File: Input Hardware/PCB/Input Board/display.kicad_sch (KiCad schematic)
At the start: 10 parts

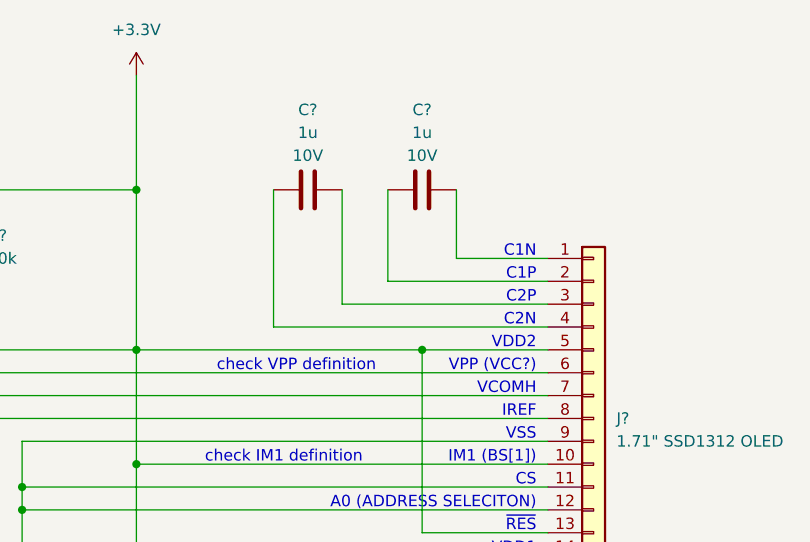
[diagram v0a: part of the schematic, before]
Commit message: images and pcb stuff
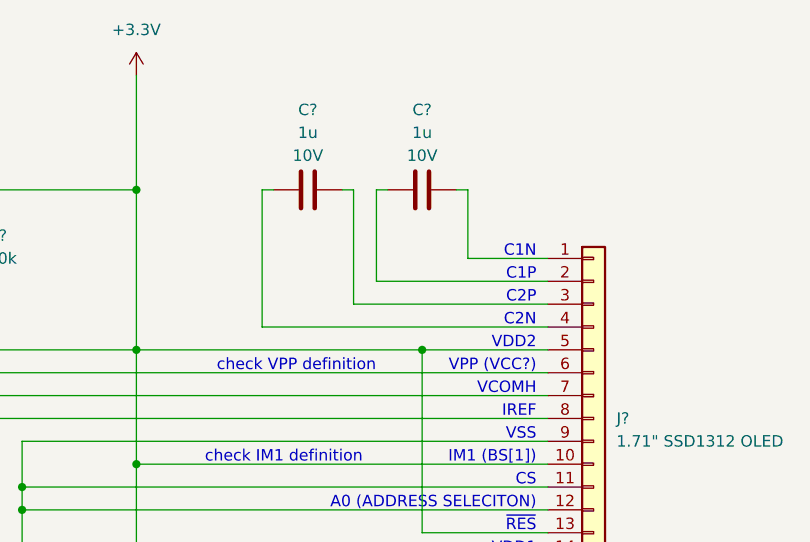
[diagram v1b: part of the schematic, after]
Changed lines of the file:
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@@
+	(wire
+		(pts
+			(xy 140.97 63.5) (xy 142.24 63.5)
+		)
+		(stroke
+			(width 0)
+			(type default)
+		)
+	)
 	(wire
 		(pts
@@
 	(wire
 		(pts
-			(xy 172.72 73.66) (xy 154.94 73.66)
+			(xy 172.72 73.66) (xy 153.67 73.66)
+		)
+		(stroke
+			(width 0)
+			(type default)
+		)
+	)
+	(wire
+		(pts
+			(xy 163.83 63.5) (xy 162.56 63.5)
 		)
 		(stroke
@@
 	(wire
 		(pts
-			(xy 162.56 71.12) (xy 172.72 71.12)
+			(xy 163.83 71.12) (xy 172.72 71.12)
+		)
+		(stroke
+			(width 0)
+			(type default)
+		)
+	)
+	(wire
+		(pts
+			(xy 153.67 63.5) (xy 154.94 63.5)
 		)
 		(stroke
@@
 	(wire
 		(pts
-			(xy 142.24 78.74) (xy 142.24 63.5)
-		)
-		(stroke
-			(width 0)
-			(type default)
-		)
-	)
-	(wire
-		(pts
-			(xy 149.86 76.2) (xy 172.72 76.2)
+			(xy 140.97 78.74) (xy 140.97 63.5)
+		)
+		(stroke
+			(width 0)
+			(type default)
+		)
+	)
+	(wire
+		(pts
+			(xy 151.13 76.2) (xy 172.72 76.2)
 		)
 		(stroke
@@
 	(wire
 		(pts
-			(xy 172.72 78.74) (xy 142.24 78.74)
+			(xy 172.72 78.74) (xy 140.97 78.74)
 		)
 		(stroke
@@
 	(wire
 		(pts
-			(xy 149.86 63.5) (xy 149.86 76.2)
-		)
-		(stroke
-			(width 0)
-			(type default)
-		)
-	)
-	(wire
-		(pts
-			(xy 154.94 73.66) (xy 154.94 63.5)
+			(xy 151.13 63.5) (xy 151.13 76.2)
+		)
+		(stroke
+			(width 0)
+			(type default)
+		)
+	)
+	(wire
+		(pts
+			(xy 153.67 73.66) (xy 153.67 63.5)
 		)
 		(stroke
@@
 	(wire
 		(pts
-			(xy 162.56 63.5) (xy 162.56 71.12)
+			(xy 163.83 63.5) (xy 163.83 71.12)
 		)
 		(stroke
@@
 		)
 		(stroke
+			(width 0)
+			(type default)
+		)
+	)
+	(wire
+		(pts
+			(xy 151.13 63.5) (xy 149.86 63.5)
+		)
+		(stroke
